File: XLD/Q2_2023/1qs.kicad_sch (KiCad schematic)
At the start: 63 parts

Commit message: mend
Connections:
- net at TWPA?.: now also L:?.; no longer L:?. (x2)
- net at L:?.: now also Eccosorb?. (x2)
- net at Eccosorb?.: now also LPF?.; no longer L:?. (x2)
- net at TJI?.: now also L:?.; no longer L:?. (x2)
- net at L:?.: no longer TJI?.
- net at TJI?.: no longer L:?.
- net at L:?.: now also TJI?.
- net at L:?.: now also Coupler?.; no longer TJI?.
- net at Eccosorb?.: now also L:?.; no longer LPF?.
- net at L:?.: no longer Eccosorb?.
- net at L:?.: now also HEMT?. (gnd); no longer TJI?.
- new net: L:?., TWPA?. (x2)
- new net: L:?., TJI?. (x3)
- new net: Eccosorb?., LPF?.
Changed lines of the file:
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@@
       (project "Q2_2023"
         (path "/9924af8b-9fcb-4325-a1dc-18dd2c4184d7" (page "7"))
-        (path "/9924af8b-9fcb-4325-a1dc-18dd2c4184d7/cbbd5daf-170b-465d-a354-f5302933c82d" (page "6"))
+        (path "/9924af8b-9fcb-4325-a1dc-18dd2c4184d7/cbbd5daf-170b-465d-a354-f5302933c82d" (page "5"))
       )
     )

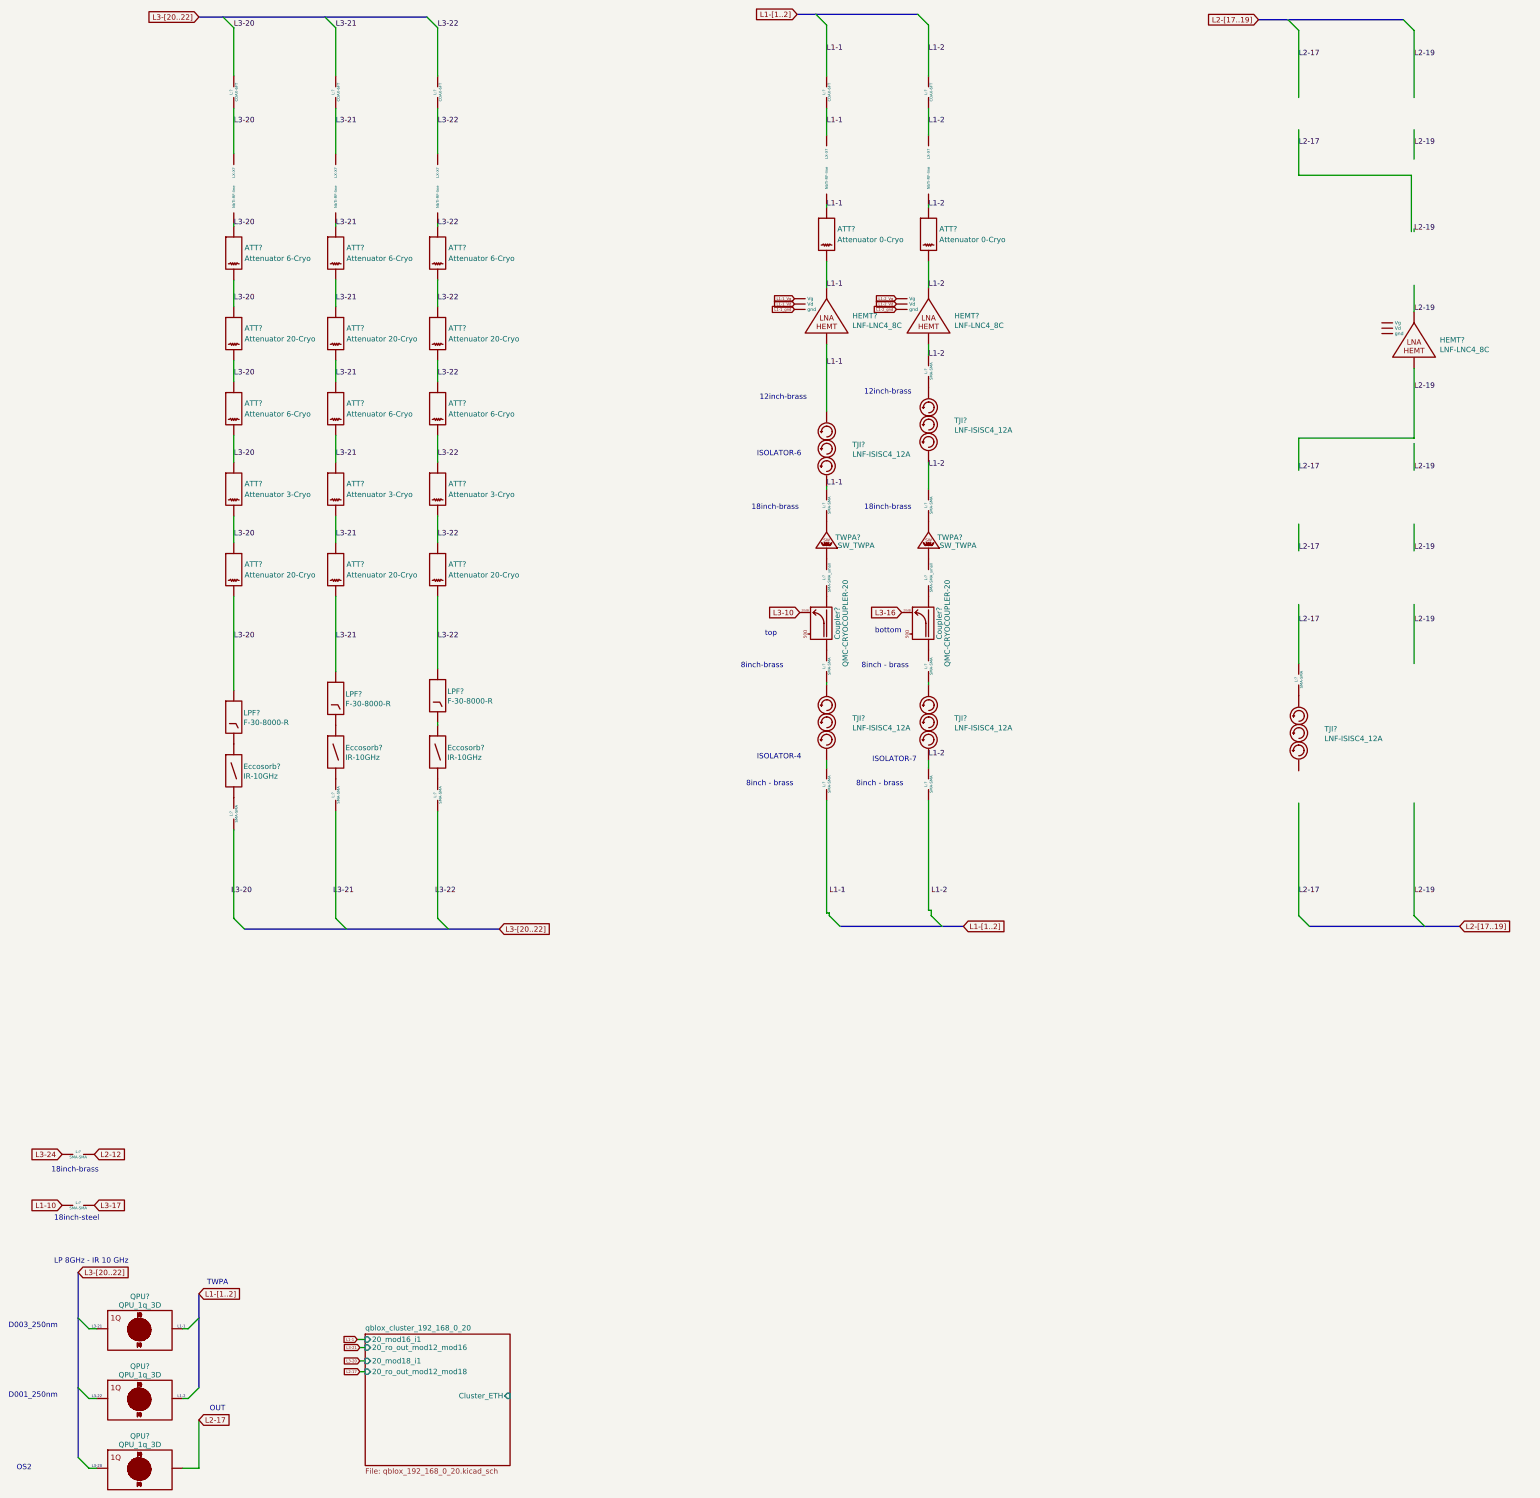
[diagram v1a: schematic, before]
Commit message: more updates
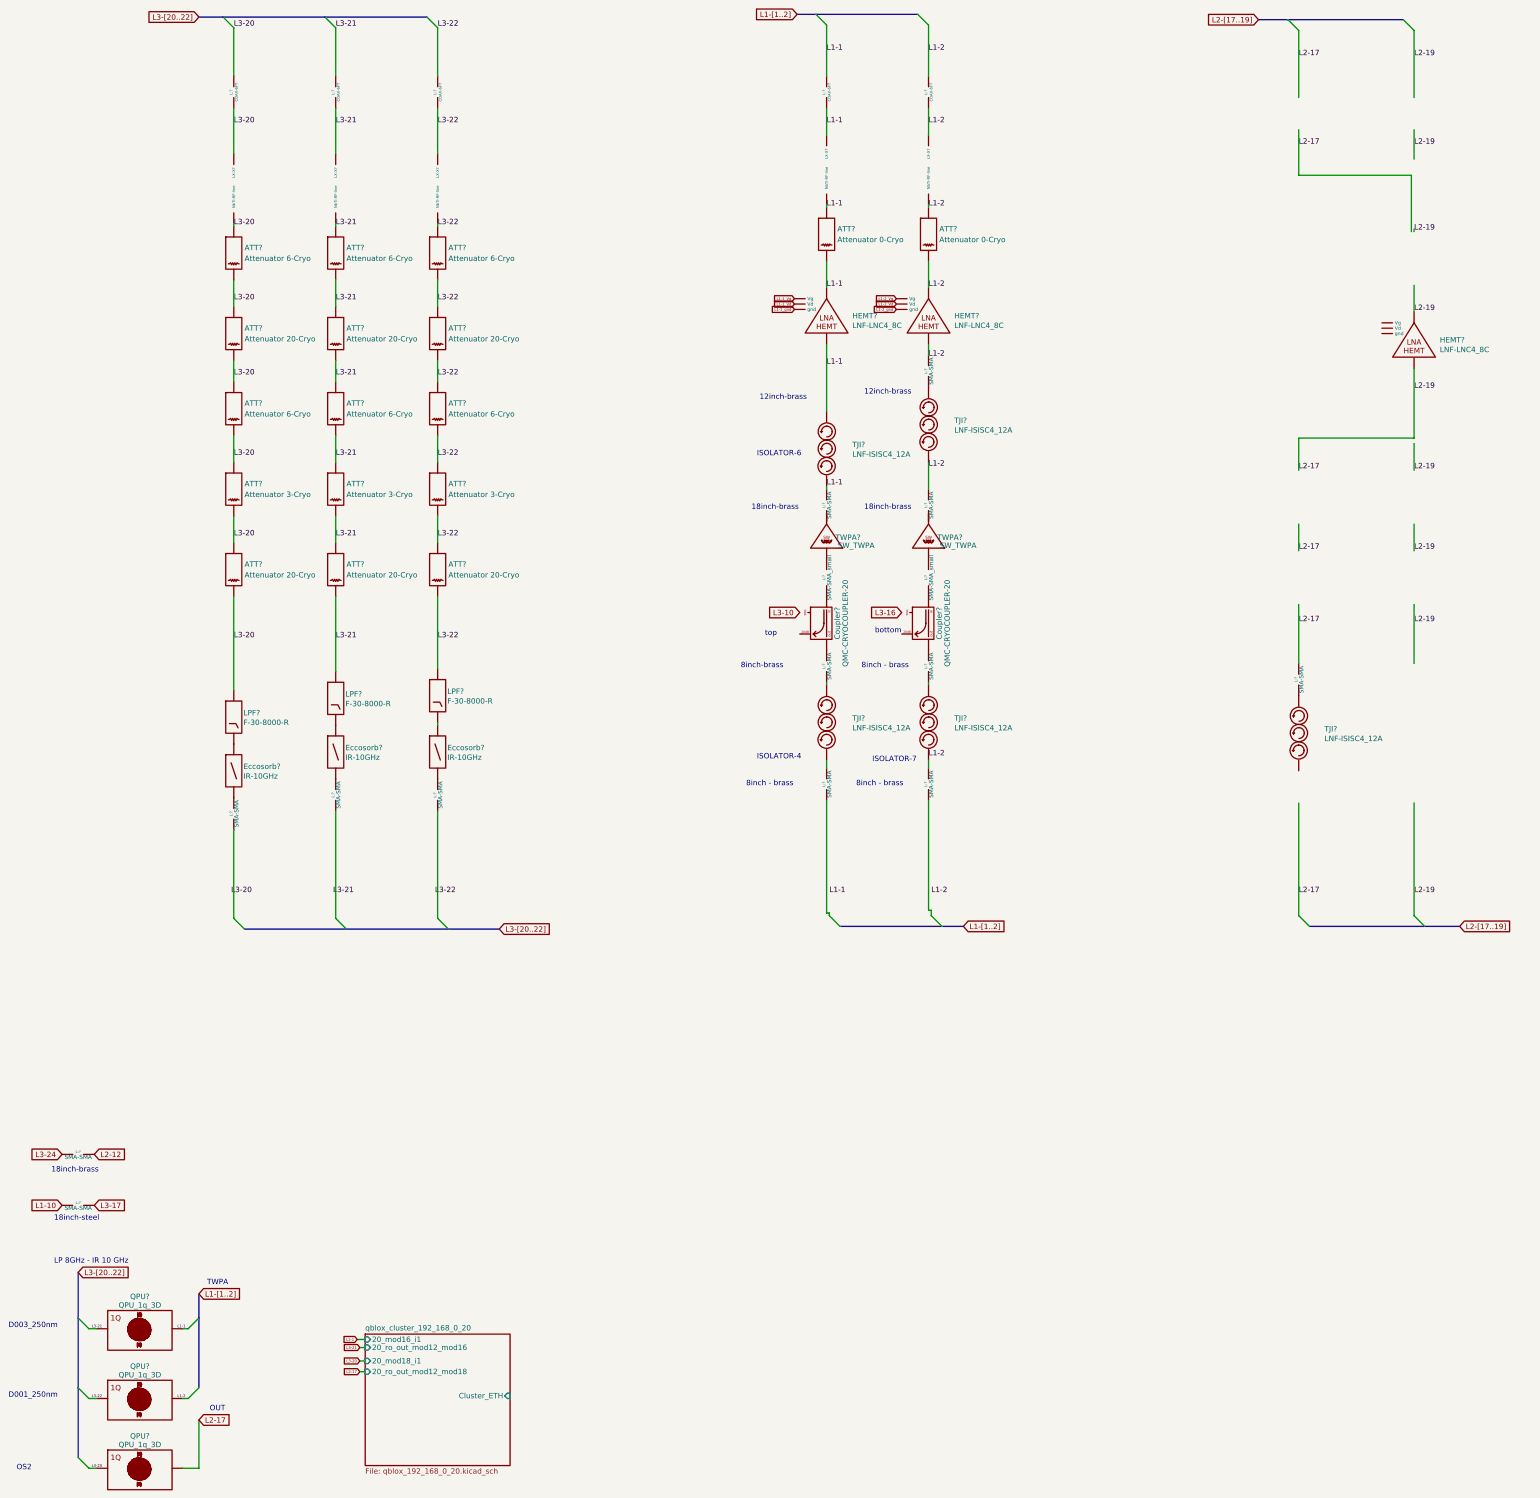
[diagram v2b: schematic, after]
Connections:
- net L3-10: no longer Coupler?.20dB
- net L3-16: no longer Coupler?.20dB
- net at L:?.: now also Eccosorb?. (x2)
- net at Eccosorb?.: now also LPF?.; no longer L:?. (x2)
- net at TJI?.: now also L:?.; no longer L:?. (x2)
- net at L:?.: no longer TJI?.
- net at TWPA?.: now also L:?.; no longer L:?.
- net at TJI?.: no longer L:?.
- net at L:?.: now also TJI?.
- net at L:?.: now also Coupler?.; no longer TJI?.
- net at Eccosorb?.: now also L:?.; no longer LPF?.
- net at L:?.: no longer Eccosorb?.
- net at L:?.: now also HEMT?. (gnd); no longer TJI?.
- new net: L:?., TJI?. (x3)
- new net: Eccosorb?., LPF?.
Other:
- moved on the sheet: TWPA?
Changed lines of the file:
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@@
     )
     (property "Value" "SMA-SMA" (at 113.665 228.6 0)
-      (effects (font (size 0.64 0.64)))
+      (effects (font (size 1 1)))
     )
     (property "Footprint" "" (at 113.03 228.6 0)
@@
     )
     (property "Value" "SMA-SMA" (at 254 160.02 0)
-      (effects (font (size 0.64 0.64)))
+      (effects (font (size 1 1)))
     )
     (property "Footprint" "" (at 253.365 160.02 0)
@@
     )
     (property "Value" "SMA-SMA" (at 341.63 201.295 0)
-      (effects (font (size 0.64 0.64)))
+      (effects (font (size 1 1)))
     )
     (property "Footprint" "" (at 340.995 201.295 0)
@@
     )
     (property "Value" "SMA-SMA" (at 229.87 226.06 0)
-      (effects (font (size 0.64 0.64)))
+      (effects (font (size 1 1)))
     )
     (property "Footprint" "" (at 229.235 226.06 0)
@@
     )
     (property "Value" "SMA-SMA" (at 254 198.12 0)
-      (effects (font (size 0.64 0.64)))
+      (effects (font (size 1 1)))
     )
     (property "Footprint" "" (at 253.365 198.12 0)
@@
     )
     (property "Value" "SMA-SMA_small" (at 229.87 177.165 0)
-      (effects (font (size 0.64 0.64)))
+      (effects (font (size 1 1)))
     )
     (property "Footprint" "" (at 229.235 177.165 0)
@@
     )
     (property "Value" "SMA-SMA" (at 254 128.27 0)
-      (effects (font (size 0.64 0.64)))
+      (effects (font (size 1 1)))
     )
     (property "Footprint" "" (at 253.365 128.27 0)
@@
     )
     (property "Value" "SMA-SMA" (at 229.87 198.12 0)
-      (effects (font (size 0.64 0.64)))
+      (effects (font (size 1 1)))
     )
     (property "Footprint" "" (at 229.235 198.12 0)
@@
     )
     (property "Value" "SMA-SMA" (at 229.87 160.02 0)
-      (effects (font (size 0.64 0.64)))
+      (effects (font (size 1 1)))
     )
     (property "Footprint" "" (at 229.235 160.02 0)
@@
     )
     (property "Value" "SMA-SMA" (at 89.535 233.045 0)
-      (effects (font (size 0.64 0.64)))
+      (effects (font (size 1 1)))
     )
     (property "Footprint" "" (at 88.9 233.045 0)
@@
     )
     (property "Value" "SMA-SMA" (at 137.795 228.6 0)
-      (effects (font (size 0.64 0.64)))
+      (effects (font (size 1 1)))
     )
     (property "Footprint" "" (at 137.16 228.6 0)
@@
     )
     (property "Value" "SMA-SMA_small" (at 254 177.165 0)
-      (effects (font (size 0.64 0.64)))
+      (effects (font (size 1 1)))
     )
     (property "Footprint" "" (at 253.365 177.165 0)
@@
     )
     (property "Value" "SMA-SMA" (at 52.07 326.39 0)
-      (effects (font (size 0.64 0.64)))
+      (effects (font (size 1 1)))
     )
     (property "Footprint" "" (at 52.07 325.755 0)
@@
     )
     (property "Value" "SMA-SMA" (at 254 226.06 0)
-      (effects (font (size 0.64 0.64)))
+      (effects (font (size 1 1)))
     )
     (property "Footprint" "" (at 253.365 226.06 0)
@@
     )
     (property "Value" "SMA-SMA" (at 52.07 314.325 0)
-      (effects (font (size 0.64 0.64)))
+      (effects (font (size 1 1)))
     )
     (property "Footprint" "" (at 52.07 313.69 0)
